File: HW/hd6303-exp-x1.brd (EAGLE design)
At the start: 100 x 80 mm, 40 parts, among them IC1 74HC245N, IC2 74HC245N, IC3 74HC245N, IC4 LM386N-1

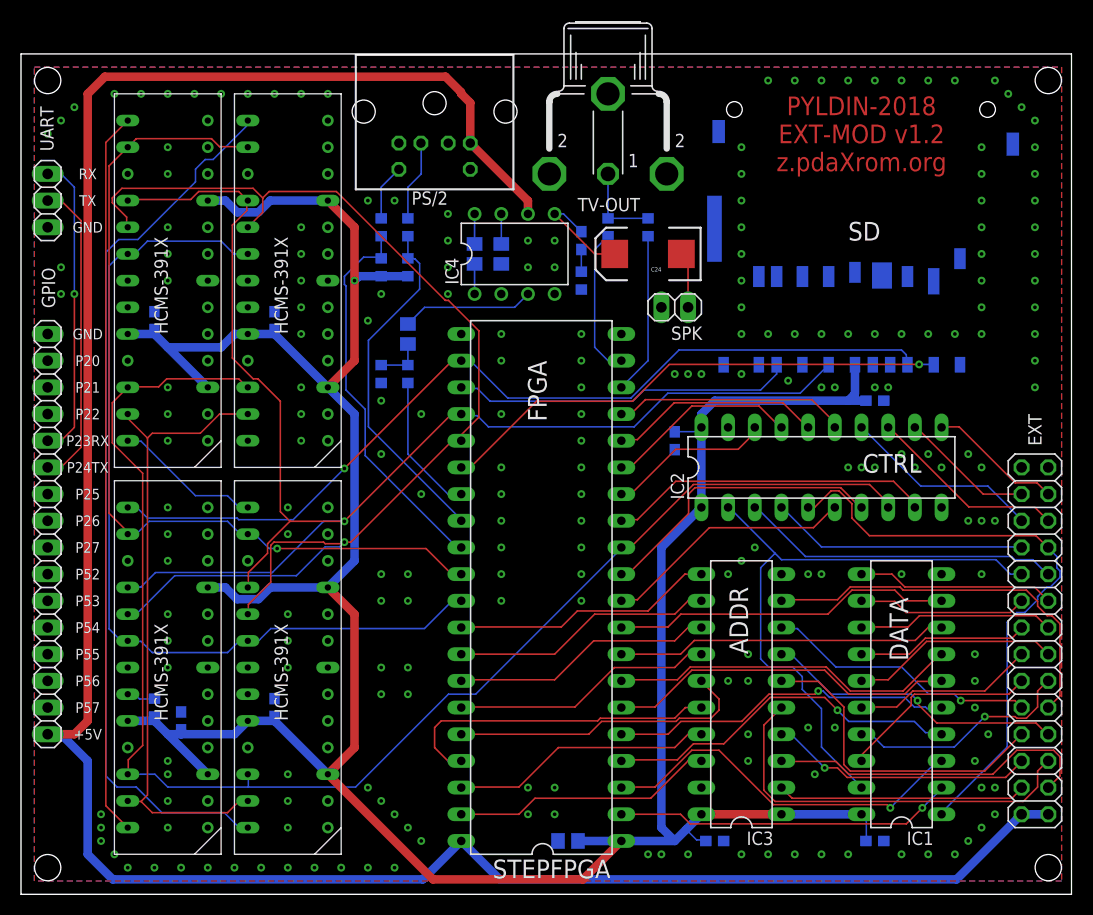
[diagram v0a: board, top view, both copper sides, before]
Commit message: released in pcb
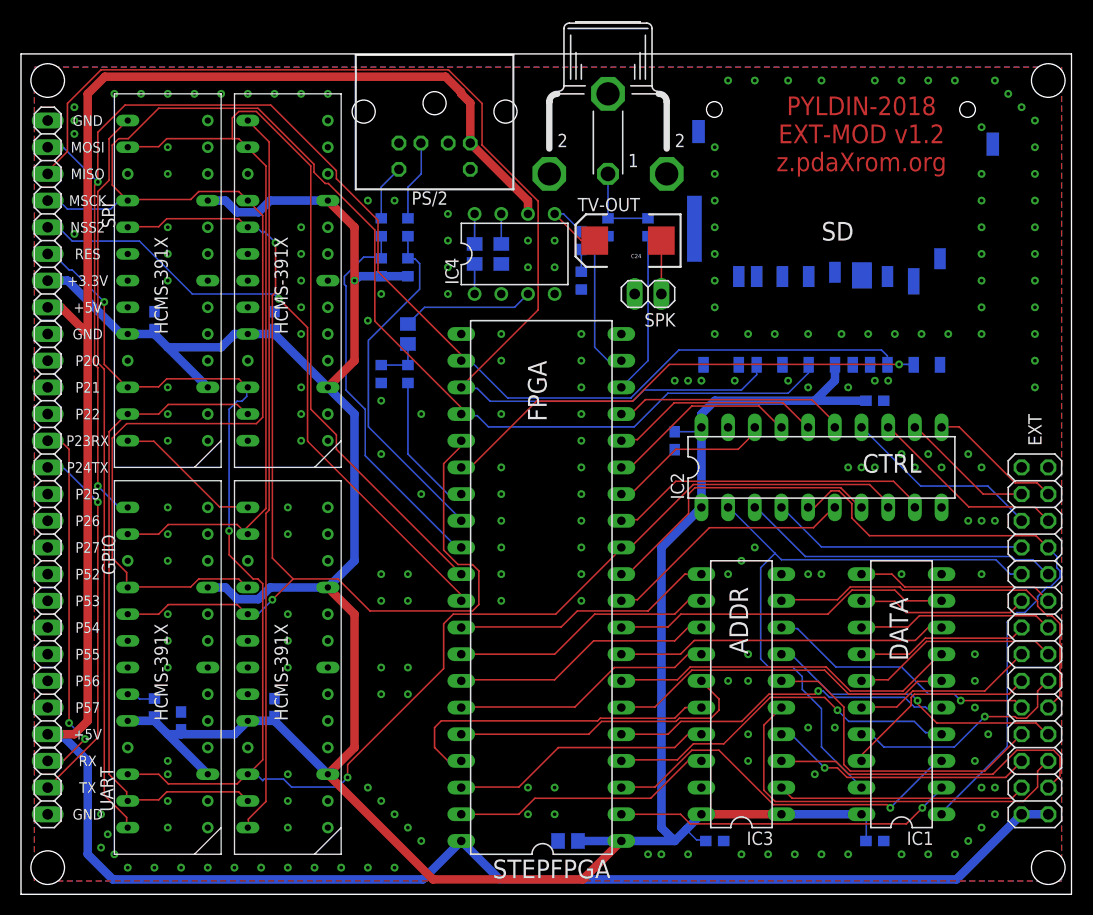
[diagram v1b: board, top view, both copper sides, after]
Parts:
- added SPI: (no value), pinhead:1X08
- moved UART 55.9 mm to (2.54, 10.2)
- moved SPK 2.84 mm to (59.7, 57.1)
- moved C24 2.29 mm to (57.8, 62.2)
- moved SDMMC 1.91 mm to (78.1, 80.0)
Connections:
- removed net BLANK: STEPFPGA.31, U$1.19, U$2.19, U$3.19, U$4.19
- new net NSS2: SPI.4, STEPFPGA.31
- net +5V: now also SPI.1
- net E_RES: now also SPI.3
- net GND: now also SPI.8, U$1.19, U$2.19, U$3.19, U$4.19
- net MISO: now also SPI.6
- net MOSI: now also SPI.7
- net MSCK: now also SPI.5
- net VCC: now also SPI.2
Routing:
- net BLANK: track 85.9 -> 0.00 mm
- net MISO: track 32.6 -> 112.7 mm
- net NSS2: track 0.00 -> 60.8 mm, vias 0 -> 1
- net MOSI: track 85.5 -> 138.3 mm, vias 1 -> 2
- net MSCK: track 135.5 -> 178.7 mm, vias 1 -> 0
- net RS: track 84.8 -> 119.5 mm, vias 1 -> 0
- net E_RES: track 138.7 -> 158.7 mm, vias 0 -> 3
- net N$3: track 85.0 -> 69.0 mm
- net VCC: track 280.2 -> 290.4 mm
- net NSS0: track 112.7 -> 104.0 mm, vias 1 -> 2
- net P23: track 29.0 -> 36.3 mm, vias 1 -> 2
- net P24: track 29.5 -> 36.6 mm, vias 0 -> 1
- net +5V: track 226.9 -> 231.7 mm
- net N$7: track 10.5 -> 8.11 mm
- net NSS1: track 49.1 -> 47.2 mm
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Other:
- board text added: "+3.3V"
- board text added: "MISO"
- board text added: "MOSI"
- board text added: "MSCK"
- board text added: "NSS2"
- board text added: "RES"
